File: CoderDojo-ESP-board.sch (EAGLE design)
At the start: 43 parts, among them IC1 ESP-12E/F, IC2 FT232RL, U1 PCA9685PW,118, U2 AMS1117-3.3, X1 PN61729-S

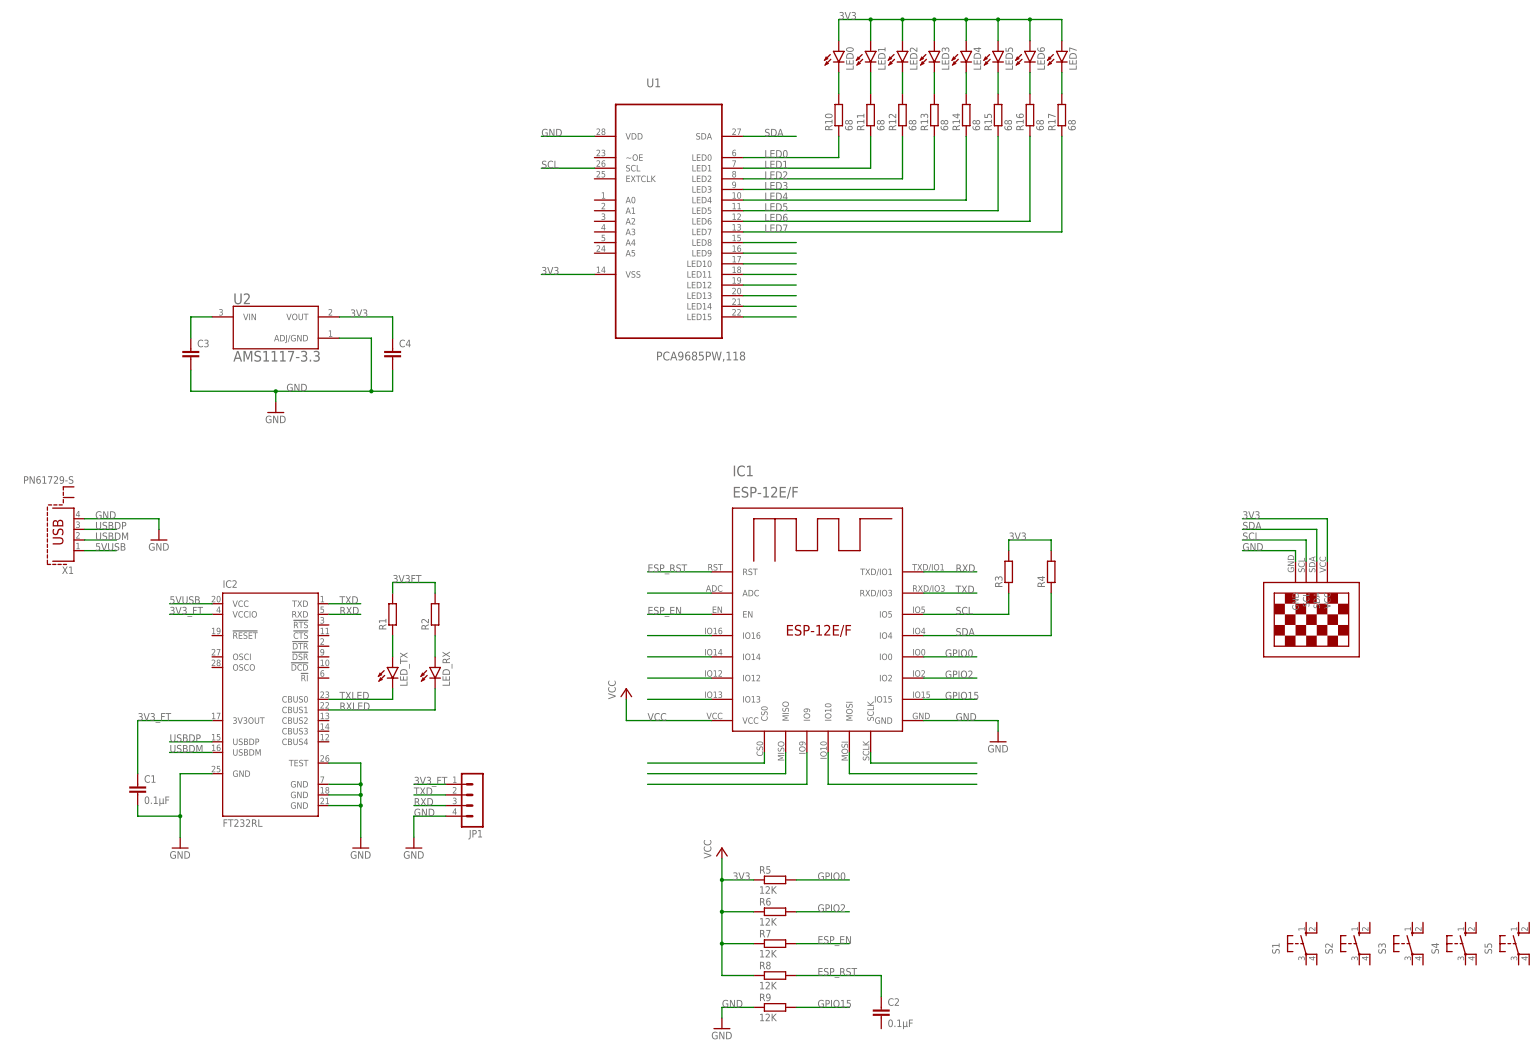
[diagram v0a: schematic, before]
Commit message: update
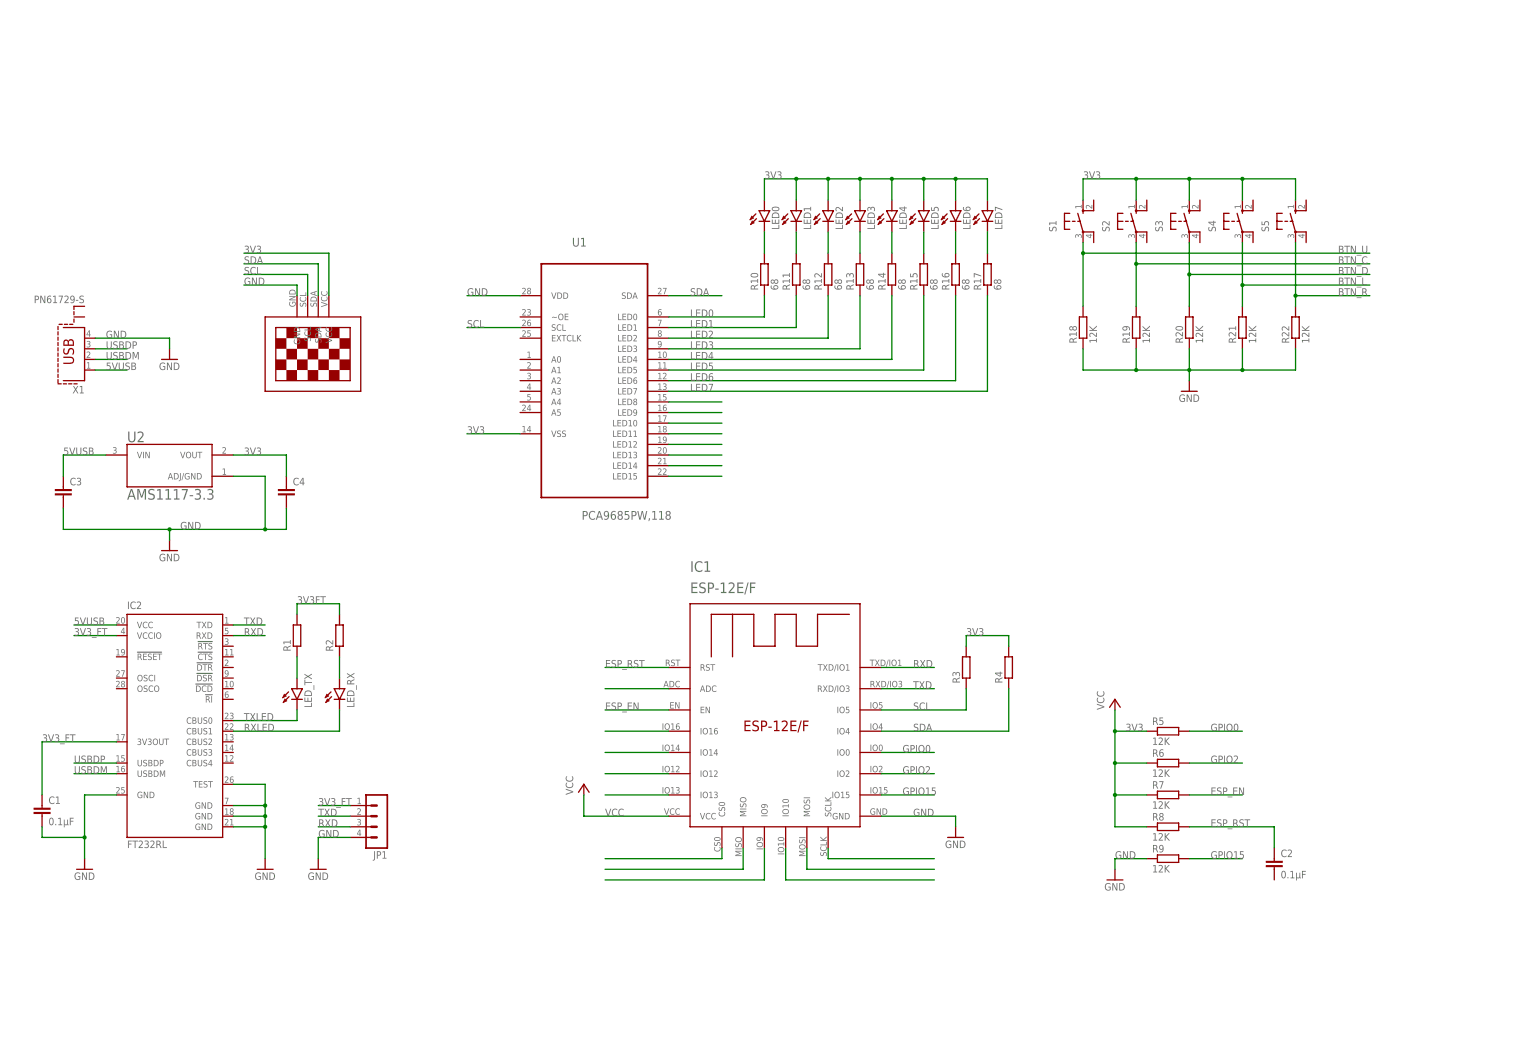
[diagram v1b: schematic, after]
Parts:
- added R18, R19, R20, R21, R22: 12K, rcl:R-EU_R0805
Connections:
- removed net N$35: C3.1, U2.VIN
- new net BTN_C: R19.2, S2.P
- new net BTN_D: R20.2, S3.P
- new net BTN_L: R21.2, S4.P
- new net BTN_R: R22.2, S5.P
- new net BTN_U: R18.2, S1.P
- net 3V3: now also S1.S, S2.S, S3.S, S4.S, S5.S
- net 5VUSB: now also C3.1, U2.VIN
- net GND: now also R18.1, R19.1, R20.1, R21.1, R22.1
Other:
- moved on the sheet: C1, C2, C3, C4, IC1, IC2, JP1, LED0, LED1, LED2, LED3, LED4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
